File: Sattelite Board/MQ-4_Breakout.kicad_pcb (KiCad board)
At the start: 2 copper layers, 21.8 x 17.3 mm, 4 parts, among them J1 Conn_01x03, U1 MQ-4

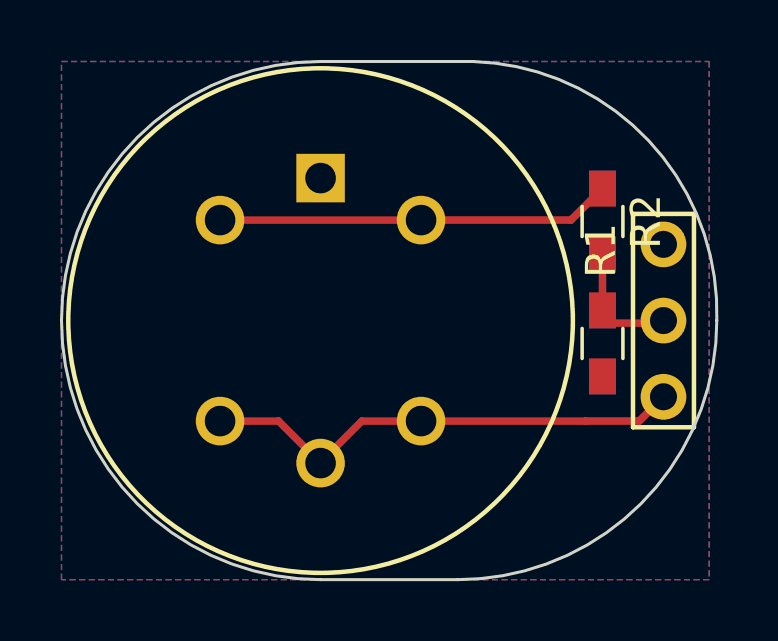
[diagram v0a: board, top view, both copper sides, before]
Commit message: Created Gerbs
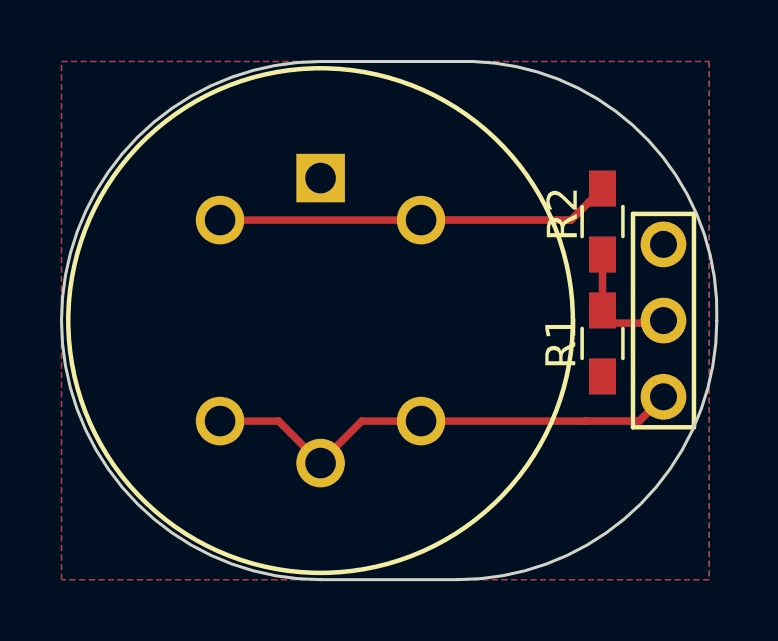
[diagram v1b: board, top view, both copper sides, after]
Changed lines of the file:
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@@
     (links 9)
     (no_connects 0)
-    (area 147.523999 94.437999 169.217849 111.810001)
+    (area 147.523999 94.437999 171.87962 111.810001)
     (thickness 1.6)
     (drawings 7)
@@
   )
   (setup
-    (last_trace_width 0.254)
+    (last_trace_width 0.25)
     (user_trace_width 0.254)
     (trace_clearance 0.2)
@@
     (visible_elements 7FFFFFFF)
     (pcbplotparams
-      (layerselection 0x00030_80000001)
+      (layerselection 0x010f0_80000001)
       (usegerberextensions false)
       (excludeedgelayer true)
@@
       (outputformat 1)
       (mirror false)
-      (drillshape 1)
+      (drillshape 0)
       (scaleselection 1)
-      (outputdirectory ""))
+      (outputdirectory Gerbs/))
   )
   (net 0 "")
@@
   (module MRDT-Headers:3x1_Header (layer F.Cu)
     (at 167.132 104.14)
-    (fp_text reference J1 (at 0.254 3.302) (layer F.SilkS) hide
+    (fp_text reference J1 (at -0.4572 3.3528) (layer F.SilkS) hide
       (effects (font (size 1 1) (thickness 0.15)))
     )
@@
     (tags "resistor 0603")
     (attr smd)
-    (fp_text reference R1 (at 3.0988 -0.0508 90) (layer F.SilkS)
+    (fp_text reference R1 (at 0.0508 -1.3716 90) (layer F.SilkS)
       (effects (font (size 1 1) (thickness 0.15)))
     )
@@
     (tags "resistor 0603")
     (attr smd)
-    (fp_text reference R2 (at 0 -1.45 270) (layer F.SilkS)
+    (fp_text reference R2 (at -0.254 1.3208 270) (layer F.SilkS)
       (effects (font (size 1 1) (thickness 0.15)))
     )
